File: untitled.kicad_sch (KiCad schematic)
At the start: 9 parts, among them J6 Input 12V-24V connector, U1 LM1117MP-3.3, U4 LM2596S-5

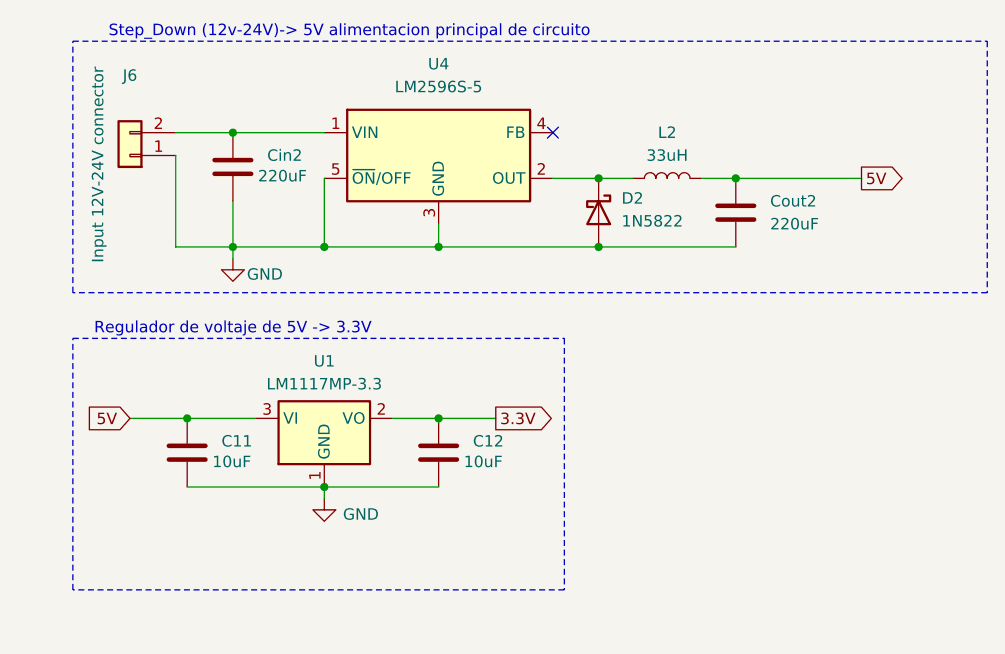
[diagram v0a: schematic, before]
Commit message: Revision 110625
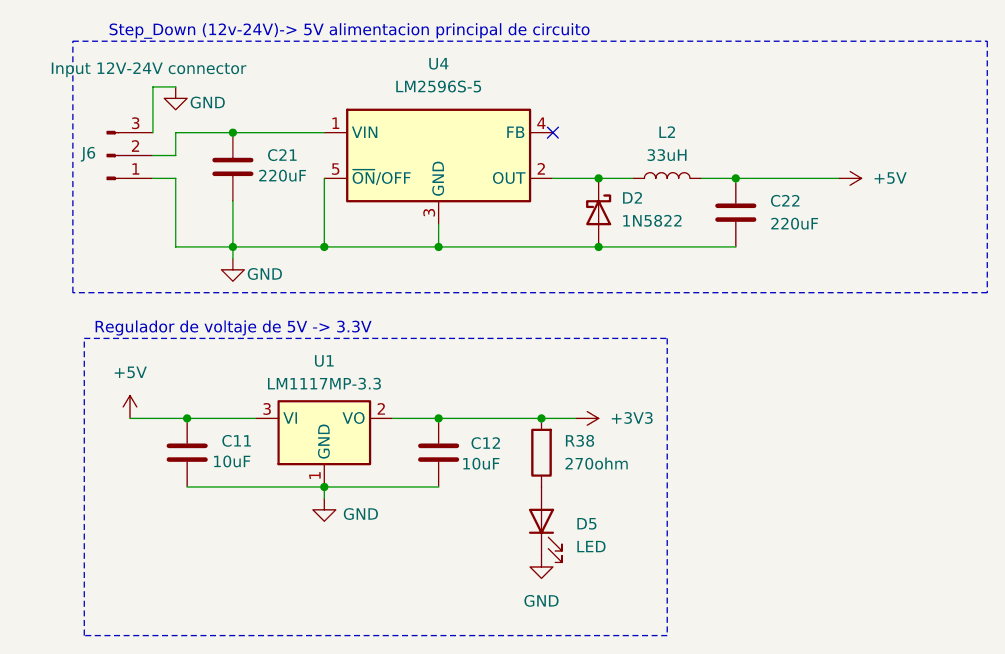
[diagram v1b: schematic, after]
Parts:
- added D5: LED, LED_SMD:LED_0805_2012Metric, symbol Device:LED
- added R38: 270ohm, Resistor_SMD:R_0805_2012Metric, symbol Device:R
- C11, C12: footprint Capacitor_SMD:C_0201_0603Metric -> Capacitor_SMD:C_0805_2012Metric; LCSC Part # (none) -> C15850
- C21: renamed from Cin2; footprint Capacitor_SMD:C_0201_0603Metric -> Capacitor_SMD:CP_Elec_10x10; LCSC Part # (none) -> C3358
- C22: renamed from Cout2; footprint Capacitor_SMD:C_0201_0603Metric -> Capacitor_SMD:CP_Elec_10x10; LCSC Part # (none) -> C3358
- D2: footprint Diode_SMD:D_0201_0603Metric -> Diode_SMD:D_SMB; LCSC Part # (none) -> C8678
- J6: symbol Connector_Generic:Conn_01x02 -> Connector:Conn_01x03_Pin
- L2: LCSC Part # (none) -> C9400
- U1: LCSC Part # (none) -> C2593
- U4: LCSC Part # (none) -> C2980820
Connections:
- net GND: now also J6.3 (Pin_3), D5.1 (K)
- net 3.3V renamed +3V3
- net +3V3: now also R38.2
- net 5V renamed +5V
- new net: D5.2 (A), R38.1
